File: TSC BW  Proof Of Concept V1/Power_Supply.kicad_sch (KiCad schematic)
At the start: 22 parts, among them J1 691312510002, Q2 AO3401A, U1 XL1509-5.0, U2 AMS1117-3.3

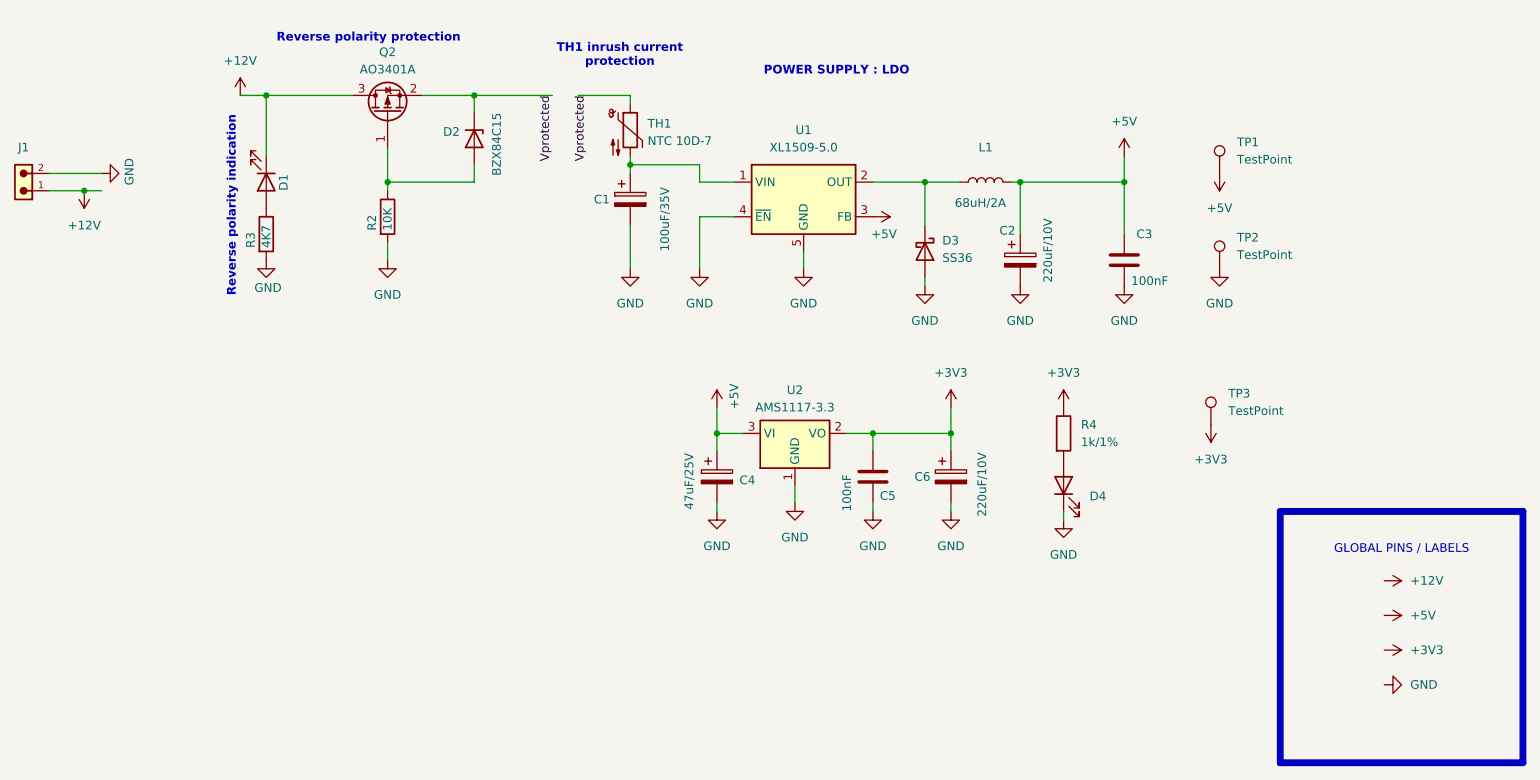
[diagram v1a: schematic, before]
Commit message: WORKING ON POC - Proof of concept
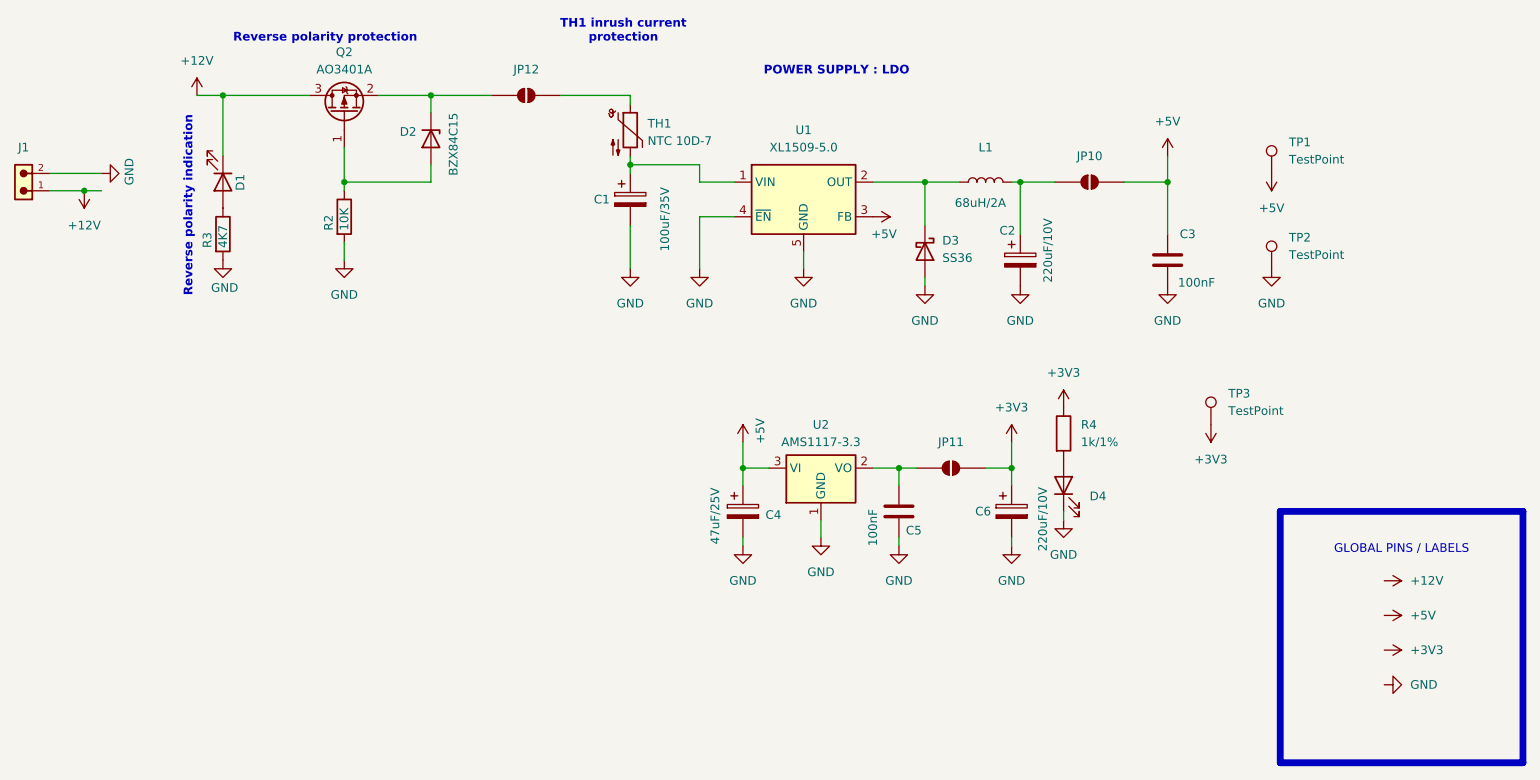
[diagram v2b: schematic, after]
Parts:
- added JP10, JP11, JP12: SolderJumper_2_Open, Jumper:SolderJumper-2_P1.3mm_Open_RoundedPad1.0x1.5mm, symbol Jumper:SolderJumper_2_Open
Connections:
- net +3V3: now also JP11.2 (B); no longer C5.1, U2.2 (VO)
- net +5V: now also JP10.2 (B); no longer C2.1, L1.2
- net Vprotected: no longer names the net of D2.3 (K), Q2.2 (S)
- net Vprotected: now also JP12.1 (A); no longer TH1.1
- new net: C2.1, JP10.1 (A), L1.2
- new net: C5.1, JP11.1 (A), U2.2 (VO)
- new net: JP12.2 (B), TH1.1
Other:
- moved on the sheet: C3, C4, C5, C6, D1, D2, Q2, R2, R3, TP1, TP2, U2
